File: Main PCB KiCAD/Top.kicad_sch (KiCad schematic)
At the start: 4 parts

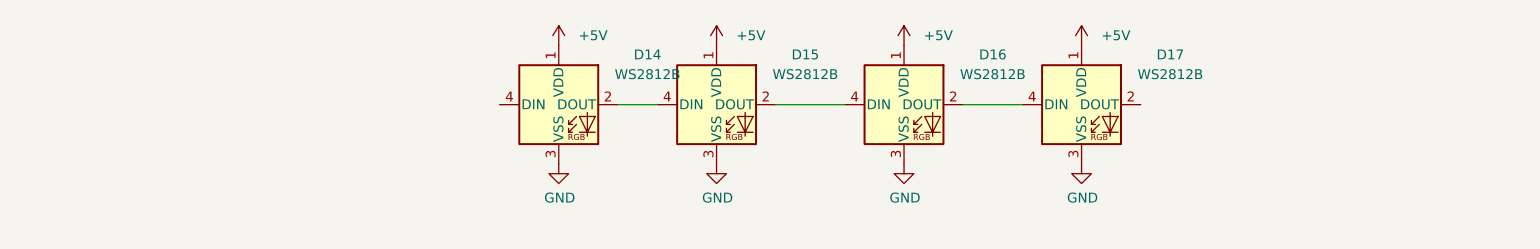
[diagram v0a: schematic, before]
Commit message: cleanup
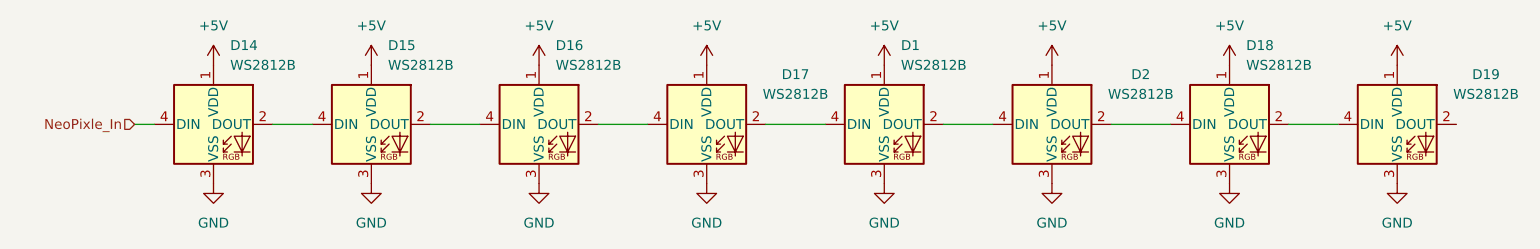
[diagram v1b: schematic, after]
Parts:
- added D1, D18, D19, D2: WS2812B, LED_SMD:LED_WS2812B_PLCC4_5.0x5.0mm_P3.2mm, symbol LED:WS2812B
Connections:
- net +5V: now also D1.1 (VDD), D18.1 (VDD), D19.1 (VDD), D2.1 (VDD)
- net GND: now also D1.3 (VSS), D18.3 (VSS), D19.3 (VSS), D2.3 (VSS)
- net at D17.2 (DOUT): now also D1.4 (DIN)
- net NeoPixle_In: now reaches D14.4 (DIN)
- new net: D1.2 (DOUT), D2.4 (DIN)
- new net: D18.2 (DOUT), D19.4 (DIN)
- new net: D18.4 (DIN), D2.2 (DOUT)
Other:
- moved on the sheet: D14, D15, D16, D17
